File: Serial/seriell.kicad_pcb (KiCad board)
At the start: 2 copper layers, 145 x 68 mm, 29 parts, among them J1 Conn_01x10_Pin, J10 Conn_01x06, J11 Conn_01x06, J12 TTL, J13 Conn_01x10_Pin, J14 Conn_01x10_Pin, J15 Conn_01x10_Pin, J16 Conn_01x10_Pin, J17 Conn_01x10_Pin, J18 Conn_01x10_Pin, J19 Bluetooth, J2 Conn_01x10_Pin, J20 Conn_01x04, J3 Conn_01x10_Pin, J30 Flash, J4 Conn_01x10_Pin, J5 Conn_01x10_Pin, J6 Conn_01x10_Pin, J7 Conn_02x04_Counter_Clockwise, J8 BT

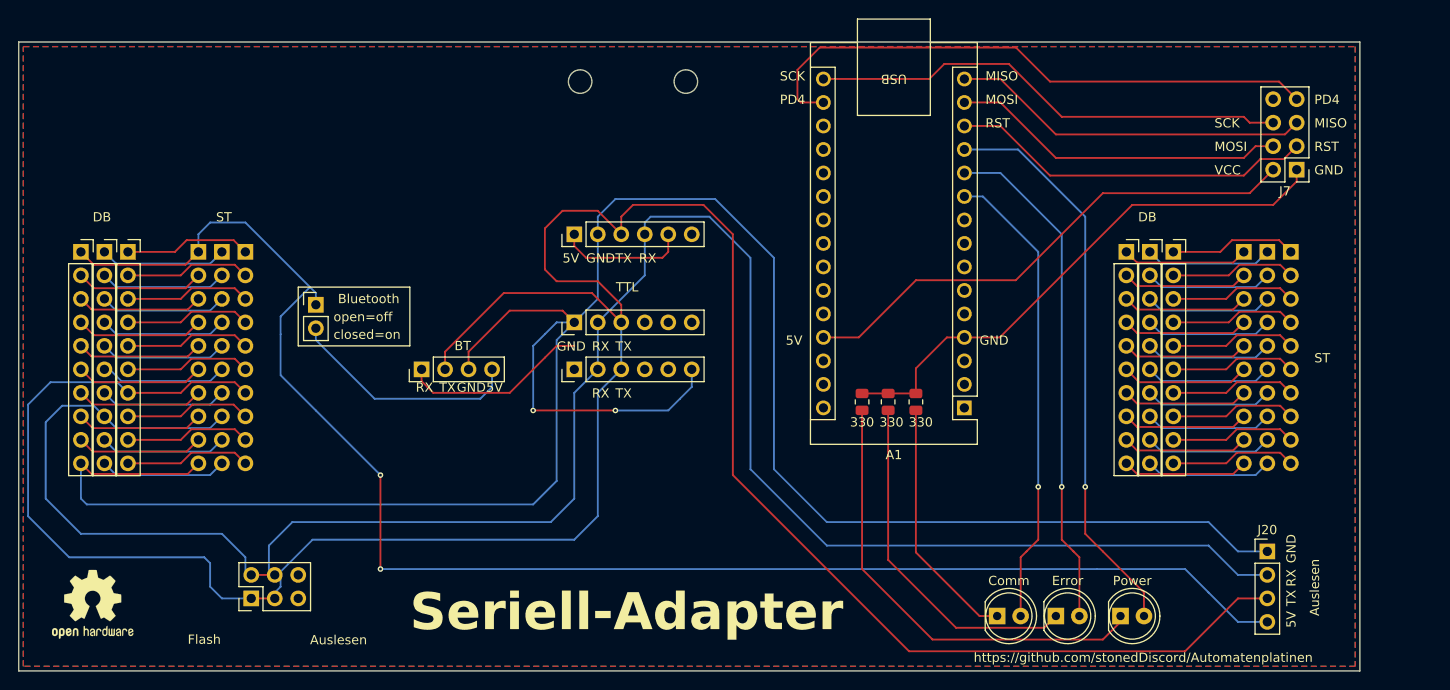
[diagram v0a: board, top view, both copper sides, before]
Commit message: serial redesign
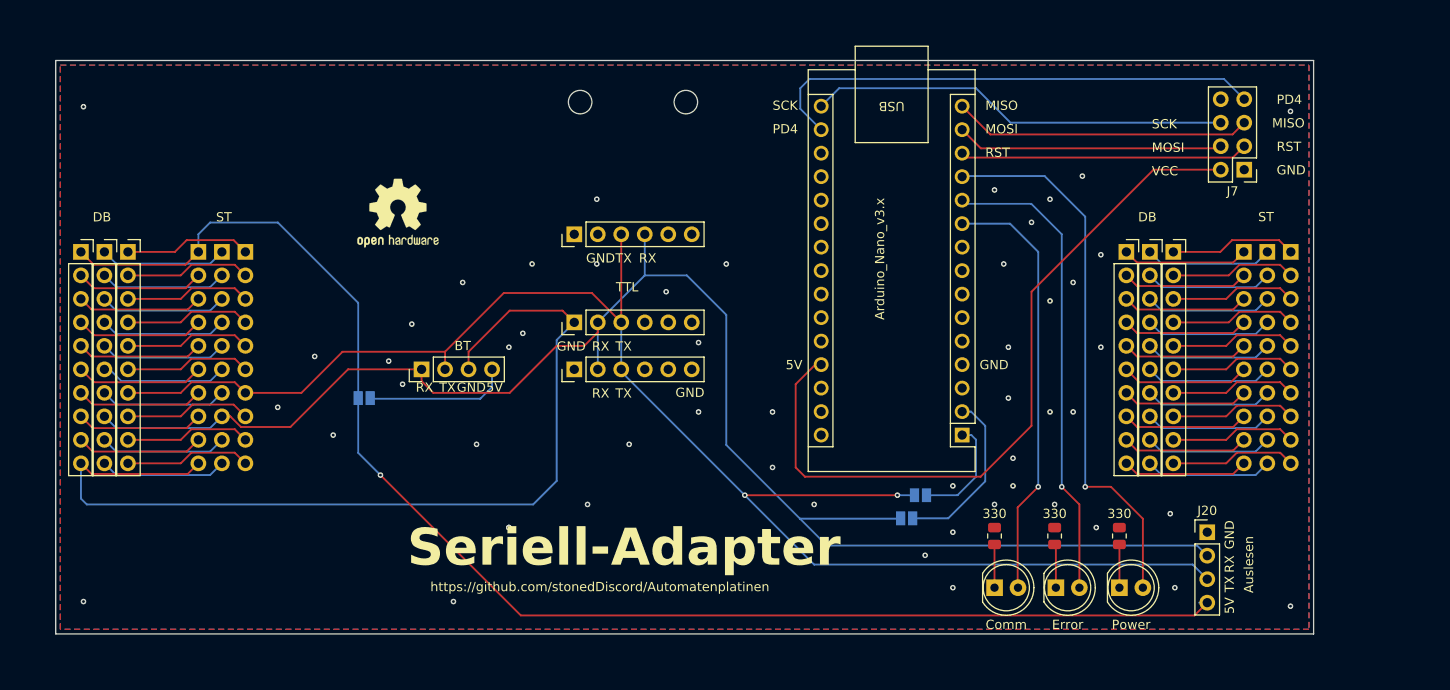
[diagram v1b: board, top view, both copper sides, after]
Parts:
- removed J19: Bluetooth, Connector_PinHeader_2.54mm:PinHeader_1x02_P2.54mm_Vertical
- removed J30: Flash, Connector_PinHeader_2.54mm:PinHeader_2x03_P2.54mm_Vertical
- added JP1: Bluetooth, Jumper:SolderJumper-2_P1.3mm_Open_Pad1.0x1.5mm, B.Cu at (116.3, 115.5)
- added JP2: RX, Jumper:SolderJumper-2_P1.3mm_Open_Pad1.0x1.5mm, B.Cu at (175.0, 128.5)
- added JP3: TX, Jumper:SolderJumper-2_P1.3mm_Open_Pad1.0x1.5mm, B.Cu at (176.5, 126.0)
- J20: value Conn_01x04 -> Auslesen
- moved REF** 53.6 mm to (120.0, 95.5)
- moved R1 31.4 mm to (198.0, 130.4)
- moved R2 23.1 mm to (191.0, 130.4)
- moved R3 16.8 mm to (184.5, 130.4)
- moved J20 6.82 mm to (207.5, 130.0)
- moved J7 5.67 mm to (211.5, 90.8)
- moved D1 3.08 mm to (184.5, 136.0)
- moved D3 3.07 mm to (198.0, 136.0)
- moved D2 3.06 mm to (191.1, 136.0)
- moved A1 2.95 mm to (181.0, 119.5)
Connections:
- net Net-(J1-Pin_1) renamed +5V
- net Net-(J10-Pin_3) renamed TX
- A1 pad 1: unconnected-(A1-D1/TX-Pad1) -> Net-(A1-D1/TX)
- A1 pad 2: unconnected-(A1-D0/RX-Pad2) -> Net-(A1-D0/RX)
- J10 pad 1: Net-(J10-Pin_1) -> unconnected-(J10-Pin_1-Pad1)
- J10 pad 4: Net-(J10-Pin_4) -> RX
- J10 pad 5: Net-(J10-Pin_1) -> unconnected-(J10-Pin_5-Pad5)
- J11 pad 2: Net-(J10-Pin_4) -> RX
- J12 pad 2: Net-(J10-Pin_4) -> RX
- J14 pad 8: Net-(J10-Pin_4) -> RX
- J2 pad 8: Net-(J10-Pin_4) -> RX
- J20 pad 2: Net-(J10-Pin_4) -> RX
- J8 pad 1: unconnected-(J8-Pin_1-Pad1) -> RX
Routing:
- net Net-(J10-Pin_4): track 226.5 -> 0.00 mm
- net GND: track 310.6 -> 103.8 mm, vias 2 -> 54
- net RX: track 0.00 -> 172.4 mm
- net TX: track 292.5 -> 168.0 mm, vias 0 -> 2
- net Net-(D3-K): track 49.7 -> 4.68 mm
- net Net-(D2-K): track 37.9 -> 4.73 mm
- net Net-(A1-+5V): track 56.1 -> 81.6 mm
- net Net-(D1-K): track 27.0 -> 4.68 mm
- net unconnected-(J8-Pin_1-Pad1): track 20.4 -> 0.00 mm
- net Net-(A1-D0/RX): track 0.00 -> 18.6 mm
- net Net-(J10-Pin_1): track 14.1 -> 0.00 mm
- net +5V: track 167.9 -> 153.9 mm, vias 2 -> 1
- net Net-(A1-D1/TX): track 0.00 -> 11.9 mm
- net Net-(J8-Pin_4): track 25.4 -> 15.1 mm
- net Net-(A1-3V3): track 63.4 -> 54.7 mm
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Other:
- board size 145 x 68 mm -> 136 x 62 mm
- board text added: "Arduino <->DB"
- board text added: "offen=aus"
- board text added: "zu=an"
- board text removed: "Auslesen"
- board text removed: "closed=on"
- board text removed: "open=off"
